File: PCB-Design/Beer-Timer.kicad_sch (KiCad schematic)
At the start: 19 parts, among them J1 Power, J2 Programmer Pins, J3 TM1637 4 Digit Display, J4 SOIC-ATtiny85-20U, J5 SOIC-2, J6 Switches, SW1 SW_SPDT, U1 MCP1700x-330xxTT, U2 ATtiny85-20S

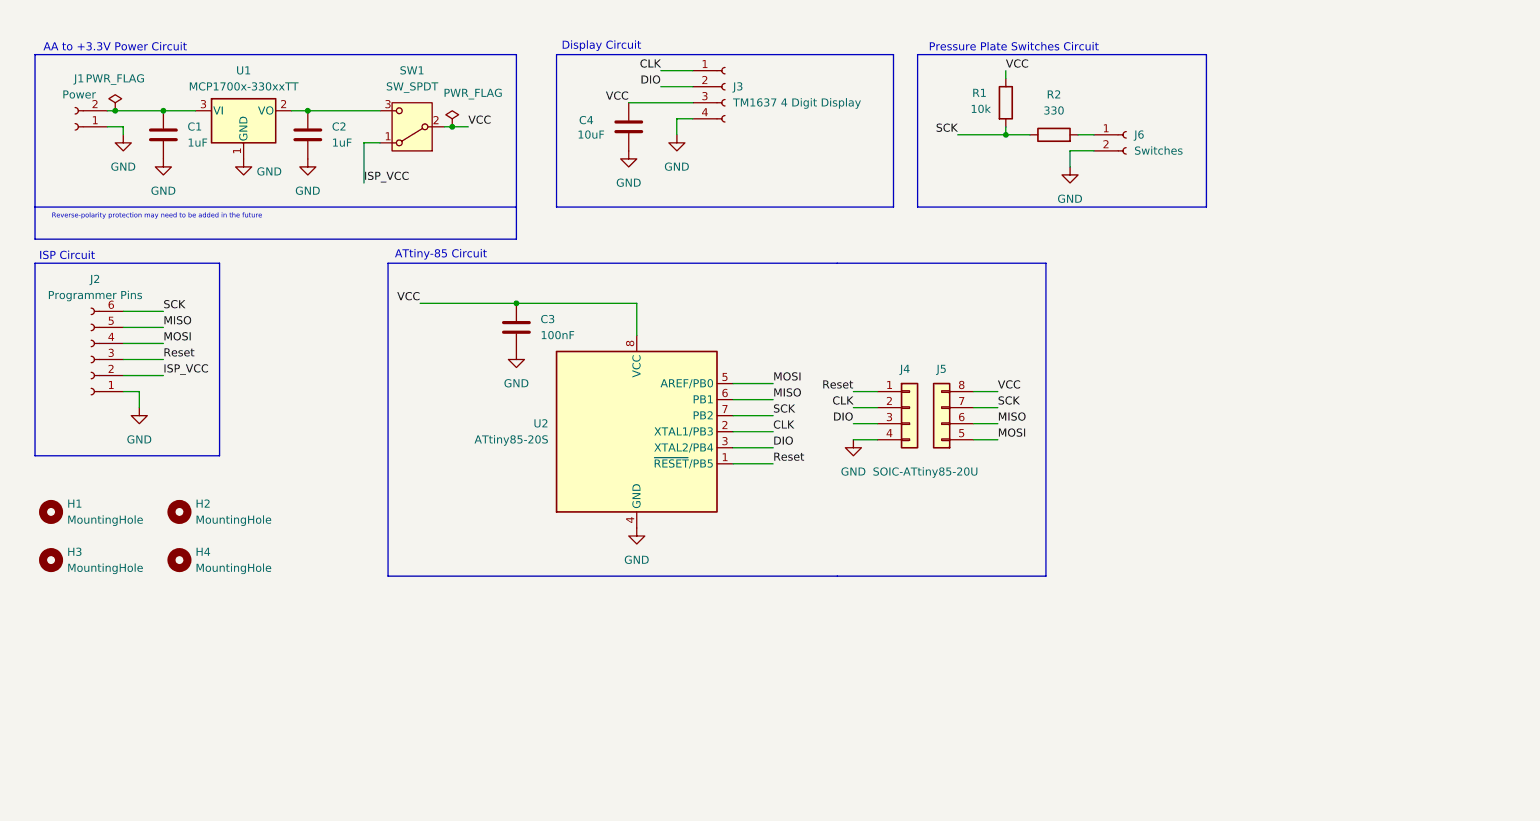
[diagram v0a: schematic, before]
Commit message: Final PCB changes
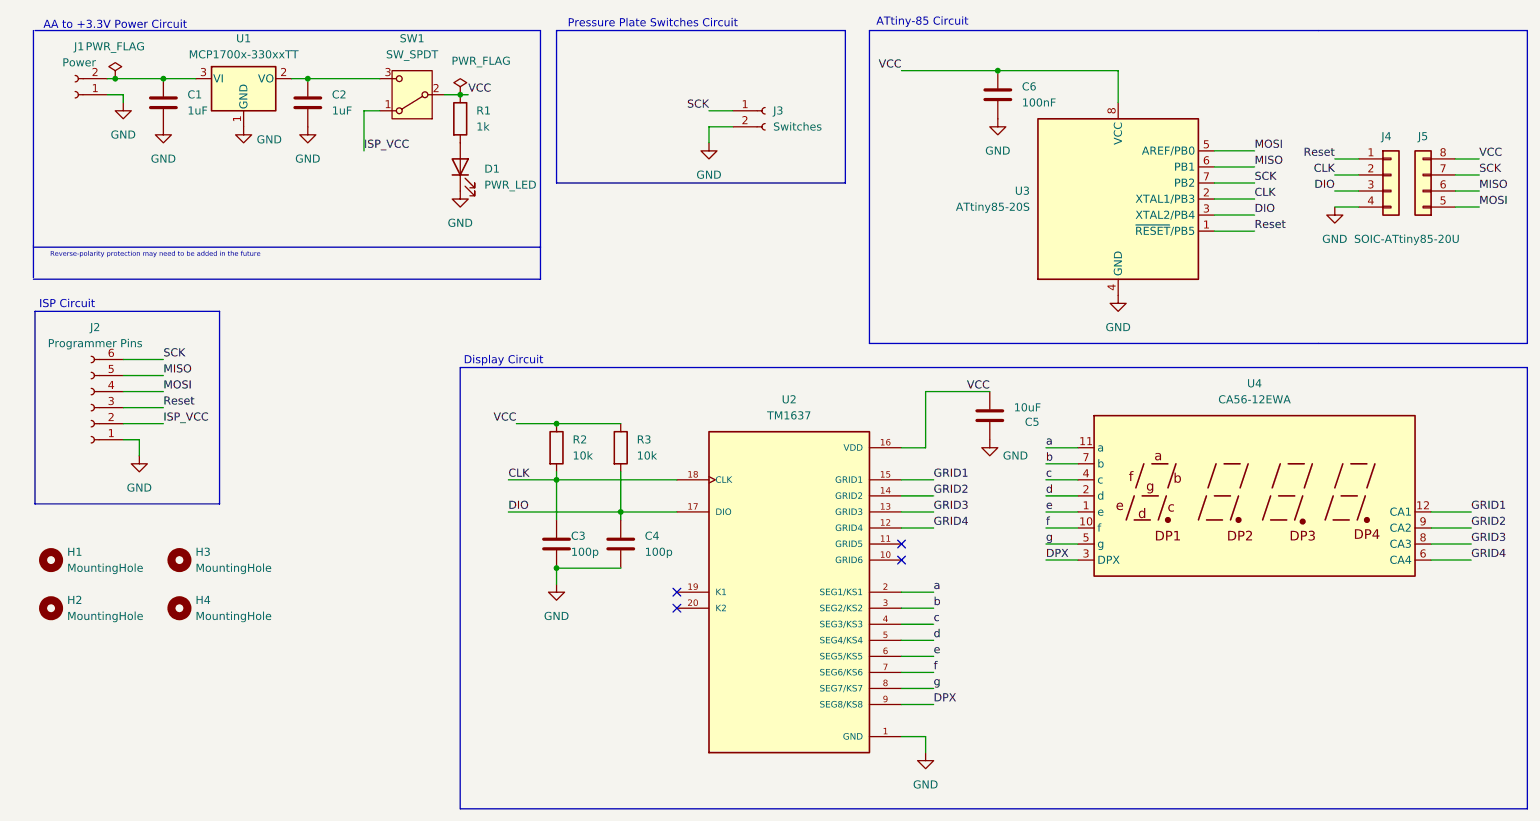
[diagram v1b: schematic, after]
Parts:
- removed J3: TM1637 4 Digit Display, Connector_PinHeader_2.54mm:PinHeader_1x04_P2.54mm_Vertical, symbol Connector:Conn_01x04_Socket
- added C3: 100p, Capacitor_SMD:C_0603_1608Metric_Pad1.08x0.95mm_HandSolder, symbol Device:C
- added C5: 10uF, Capacitor_SMD:C_0603_1608Metric_Pad1.08x0.95mm_HandSolder, symbol Device:C
- added D1: PWR_LED, LED_SMD:LED_0603_1608Metric_Pad1.05x0.95mm_HandSolder, symbol Device:LED
- added R3: 10k, Resistor_SMD:R_0603_1608Metric_Pad0.98x0.95mm_HandSolder, symbol Device:R
- added U2: TM1637, Package_SO:SOP-20_7.5x12.8mm_P1.27mm, symbol TM1637:TM1637
- added U4: CA56-12EWA, Display_7Segment:CA56-12EWA, symbol Display_Character:CA56-12EWA
- C4: value 10uF -> 100p
- R1: value 10k -> 1k
- R2: value 330 -> 10k
- renumbered C3 to C6, H3 to H2, H2 to H3, J6 to J3, U2 to U3
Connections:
- net CLK: now also R2.2, C3.1, U2.18 (CLK)
- net DIO: now also C4.1, R3.2, U2.17 (DIO)
- net GND: now also C3.2, C5.1, D1.1 (K), U2.1 (GND)
- net SCK: now also J3.1 (Pin_1); no longer R1.2, R2.1
- net VCC: now also R2.1, C5.2, R3.1, U2.16 (VDD); no longer C4.1
- new net: D1.2 (A), R1.2
- new net DPX: U2.9 (SEG8/KS8), U4.3 (DPX)
- new net GRID1: U2.15 (GRID1), U4.12 (CA1)
- new net GRID2: U2.14 (GRID2), U4.9 (CA2)
- new net GRID3: U2.13 (GRID3), U4.8 (CA3)
- new net GRID4: U2.12 (GRID4), U4.6 (CA4)
- new net a: U2.2 (SEG1/KS1), U4.11 (a)
- new net b: U2.3 (SEG2/KS2), U4.7 (b)
- new net c: U2.4 (SEG3/KS3), U4.4 (c)
- new net d: U2.5 (SEG4/KS4), U4.2 (d)
- new net e: U2.6 (SEG5/KS5), U4.1 (e)
- new net f: U2.7 (SEG6/KS6), U4.10 (f)
- new net g: U2.8 (SEG7/KS7), U4.5 (g)
- no-connect marks 0 -> 4
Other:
- moved on the sheet: C1, C2, C6, H1, H2, H3, H4, J1, J2, J3, J4, J5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
